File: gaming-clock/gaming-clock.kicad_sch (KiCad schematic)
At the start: 28 parts, among them J1 USB_C_Receptacle_USB2.0, J2 Barrel_Jack_Switch, Q1 Q_Photo_NPN_CE, Q2 PMOS, Q3 PMOS, U1 ESP32-C3-WROOM-02, U2 LM1117GS-3.3

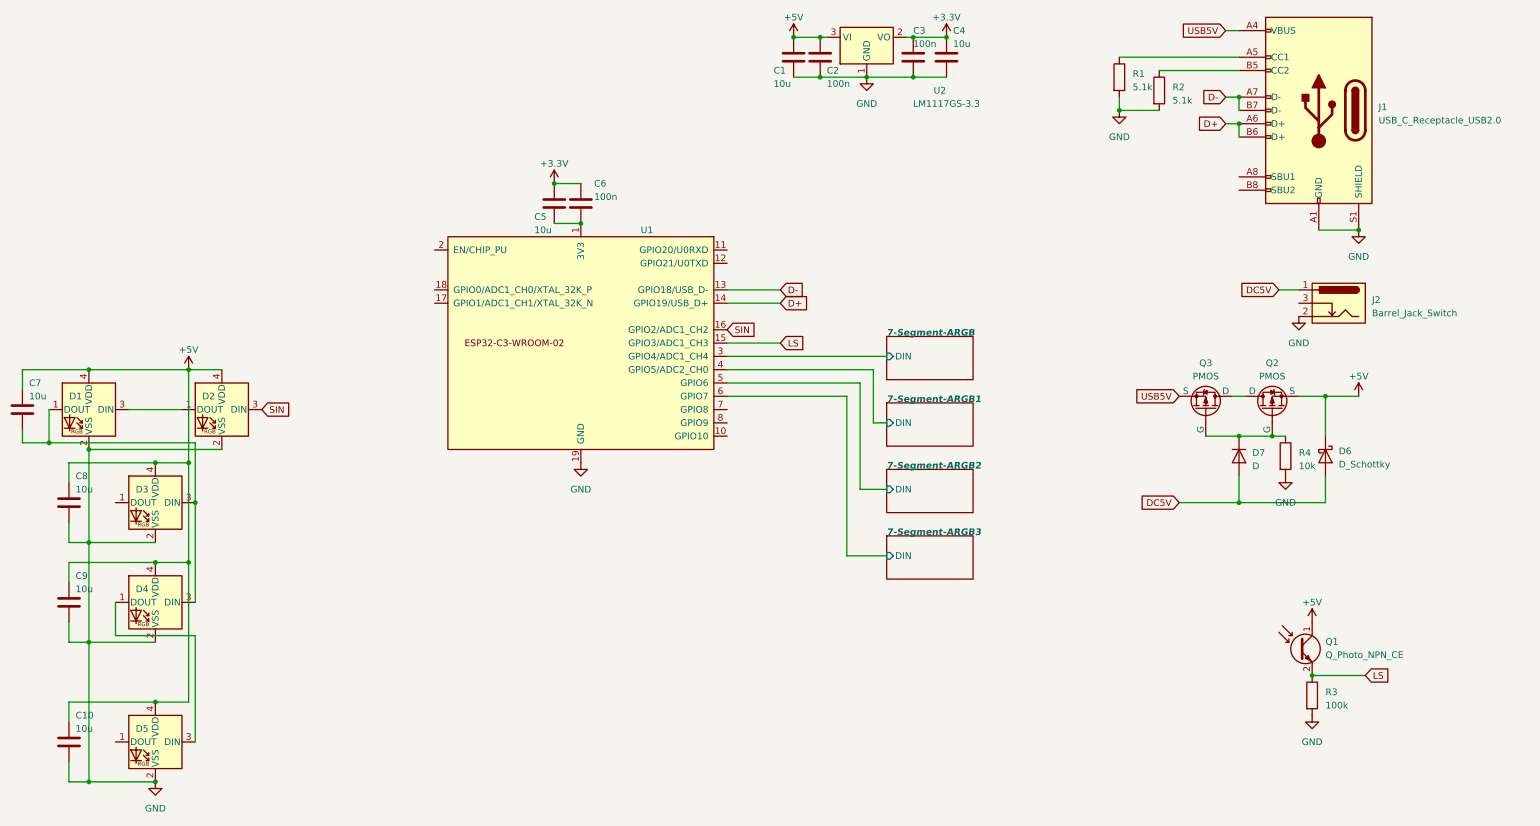
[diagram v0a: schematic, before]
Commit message: fin
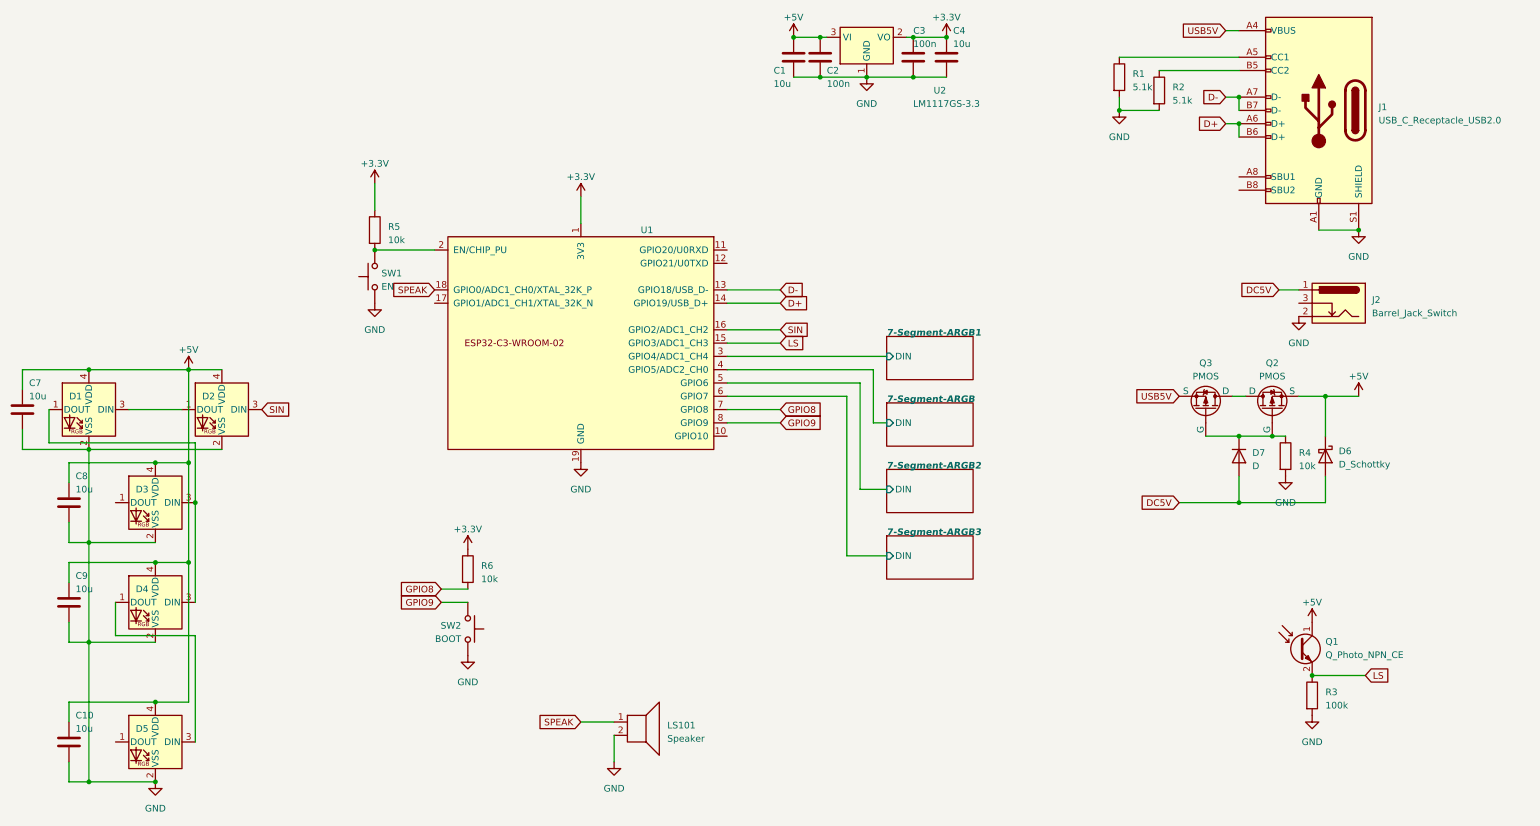
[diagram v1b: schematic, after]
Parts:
- removed C5: 10u, Capacitor_SMD:C_0603_1608Metric_Pad1.08x0.95mm_HandSolder, symbol Device:C
- removed C6: 100n, Capacitor_SMD:C_0603_1608Metric_Pad1.08x0.95mm_HandSolder, symbol Device:C
- added LS101: Speaker, Buzzer_Beeper:Buzzer_TDK_PS1240P02BT_D12.2mm_H6.5mm, symbol Device:Speaker
- added R5, R6: 10k, Resistor_SMD:R_0603_1608Metric_Pad0.98x0.95mm_HandSolder, symbol Device:R
- added SW1: EN, Button_Switch_SMD:SW_Push_1P1T_NO_Vertical_Wuerth_434133025816, symbol Switch:SW_Push
- added SW2: BOOT, Button_Switch_SMD:SW_Push_1P1T_NO_Vertical_Wuerth_434133025816, symbol Switch:SW_Push
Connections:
- net +3.3V: now also U1.1 (3V3), R5.1, R6.1
- net 7-Segment-ARGB/DIN: now also U1.4 (GPIO5/ADC2_CH0); no longer U1.3 (GPIO4/ADC1_CH4)
- net 7-Segment-ARGB1/DIN: now also U1.3 (GPIO4/ADC1_CH4); no longer U1.4 (GPIO5/ADC2_CH0)
- net GND: now also C7.2, LS101.2, SW1.2, SW2.2
- net SPEAK: now reaches U1.18 (GPIO0/ADC1_CH0/XTAL_32K_P)
- net SPEAK: now also LS101.1
- net at U1.2 (EN/CHIP_PU): now also R5.2, SW1.1
- net GPIO8: now reaches U1.7 (GPIO8)
- net GPIO8: now also R6.2
- net GPIO9: now reaches U1.8 (GPIO9)
- net GPIO9: now also SW2.1
- net at D1.1 (DOUT), D3.3 (DIN), D4.3 (DIN): no longer C7.2
